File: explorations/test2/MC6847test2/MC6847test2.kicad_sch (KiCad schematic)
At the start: 16 parts, among them J1 RCA, Q1 2N2222, Q2 2N2222, U1 74LS04, U2 MC6847P, Y1 3.57945 MHz

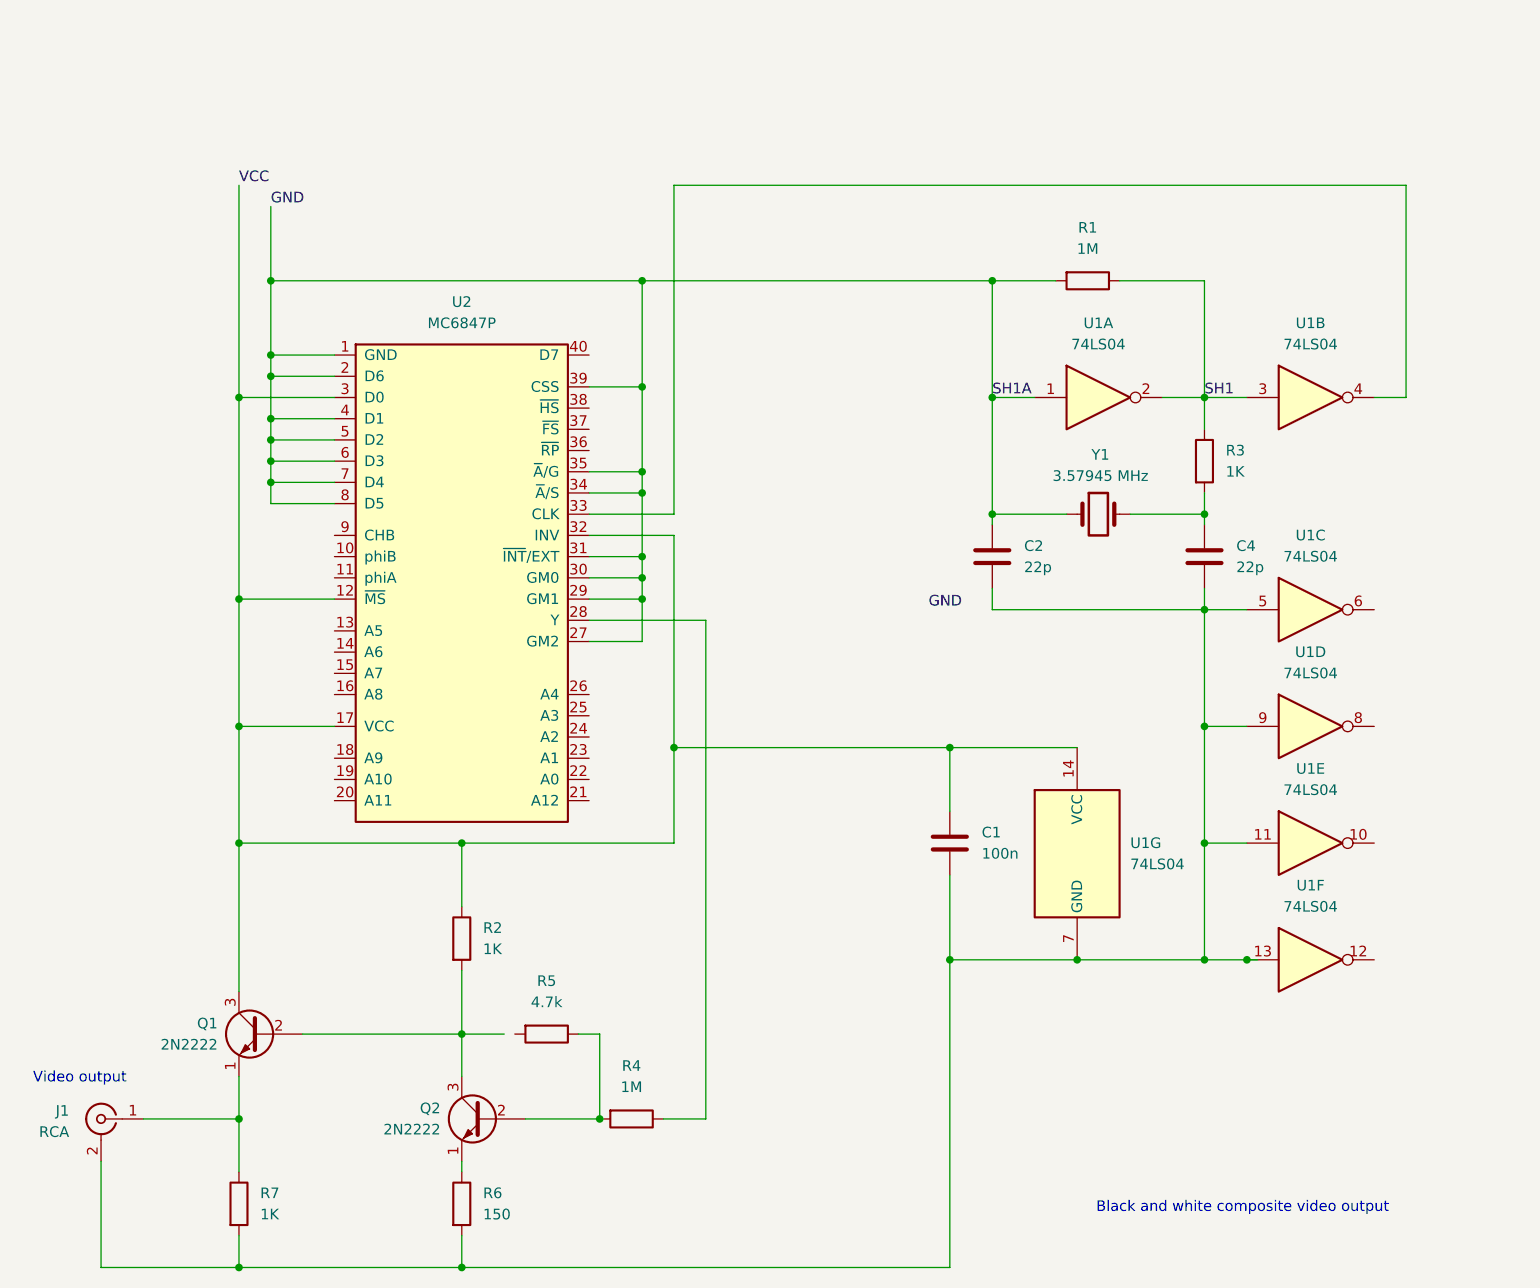
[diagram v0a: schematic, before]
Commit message: update test2 & test3
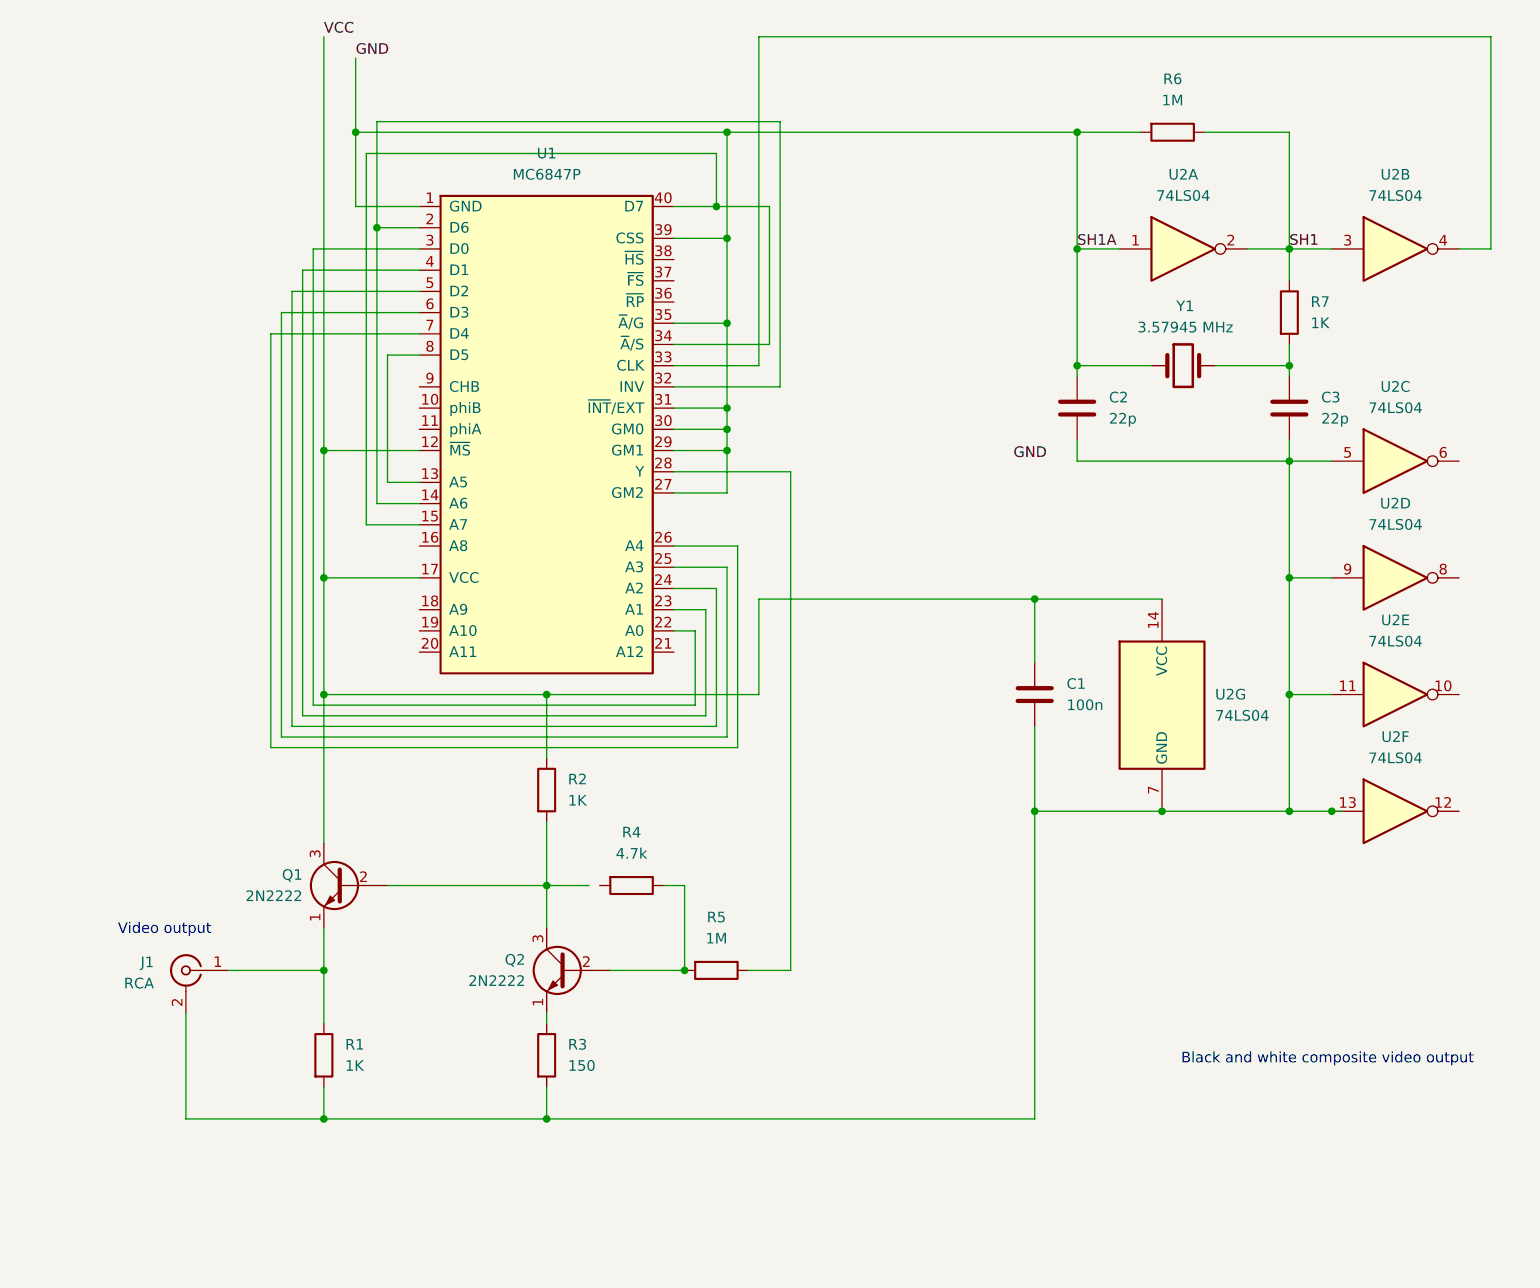
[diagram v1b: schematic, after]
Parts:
- removed C4: 22p, Capacitor_THT:C_Disc_D3.0mm_W1.6mm_P2.50mm, symbol Device:C
- removed U1: 74LS04, symbol 74xx:74LS04
- removed U2: MC6847P, Package_DIP:DIP-40_W15.24mm, symbol myGPU:MC6847P
- added C3: 22p, Capacitor_THT:C_Disc_D3.0mm_W1.6mm_P2.50mm, symbol Device:C
- added U1: MC6847P, Package_DIP:DIP-40_W15.24mm, symbol myGPU:MC6847P
- added U2: 74LS04, symbol 74xx:74LS04
- R1: value 1M -> 1K
- R3: value 1K -> 150
- R4: value 1M -> 4.7k
- R5: value 4.7k -> 1M
- R6: value 150 -> 1M
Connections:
- net GND: now also R6.2, U1.1 (GND), U1.27 (GM2), U1.29 (GM1), U1.30 (GM0), U1.31 (~{INT}/EXT), U1.35 (~{A}/G), U1.39 (CSS), U2.1; no longer R1.2
- net SH1: now also R6.1, R7.1, U2.2, U2.3; no longer R1.1, R3.1
- net VCC: now also U1.12 (~{MS}), U1.17 (VCC), U2.14 (VCC)
- net at Q2.1 (E): now also R3.1; no longer R6.1
- net at C1.2, C2.2, J1.2 (Ext): now also R1.2, R3.2, C3.2, U2.11, U2.13, U2.5, U2.7 (GND), U2.9; no longer R6.2, R7.2
- net at Y1.2: now also R7.2, C3.1; no longer R3.2
- net at R4.1: now also Q2.2 (B), R5.2
- net at J1.1 (In), Q1.1 (E): now also R1.1; no longer R7.1
- new net: U1.33 (CLK), U2.4
- new net: R5.1, U1.28 (Y)
- new net: U1.13 (A5), U1.8 (D5)
- new net: U1.14 (A6), U1.2 (D6), U1.32 (INV)
- new net: U1.15 (A7), U1.34 (~{A}/S), U1.40 (D7)
- new net: U1.22 (A0), U1.3 (D0)
- new net: U1.23 (A1), U1.4 (D1)
- new net: U1.24 (A2), U1.5 (D2)
- new net: U1.25 (A3), U1.6 (D3)
- new net: U1.26 (A4), U1.7 (D4)
- now unconnected: R4.2
